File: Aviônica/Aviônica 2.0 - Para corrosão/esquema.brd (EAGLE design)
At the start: 128 x 64.1 mm, 15 parts, among them M1 WIRELESS-NRF24L01-PA-EXT

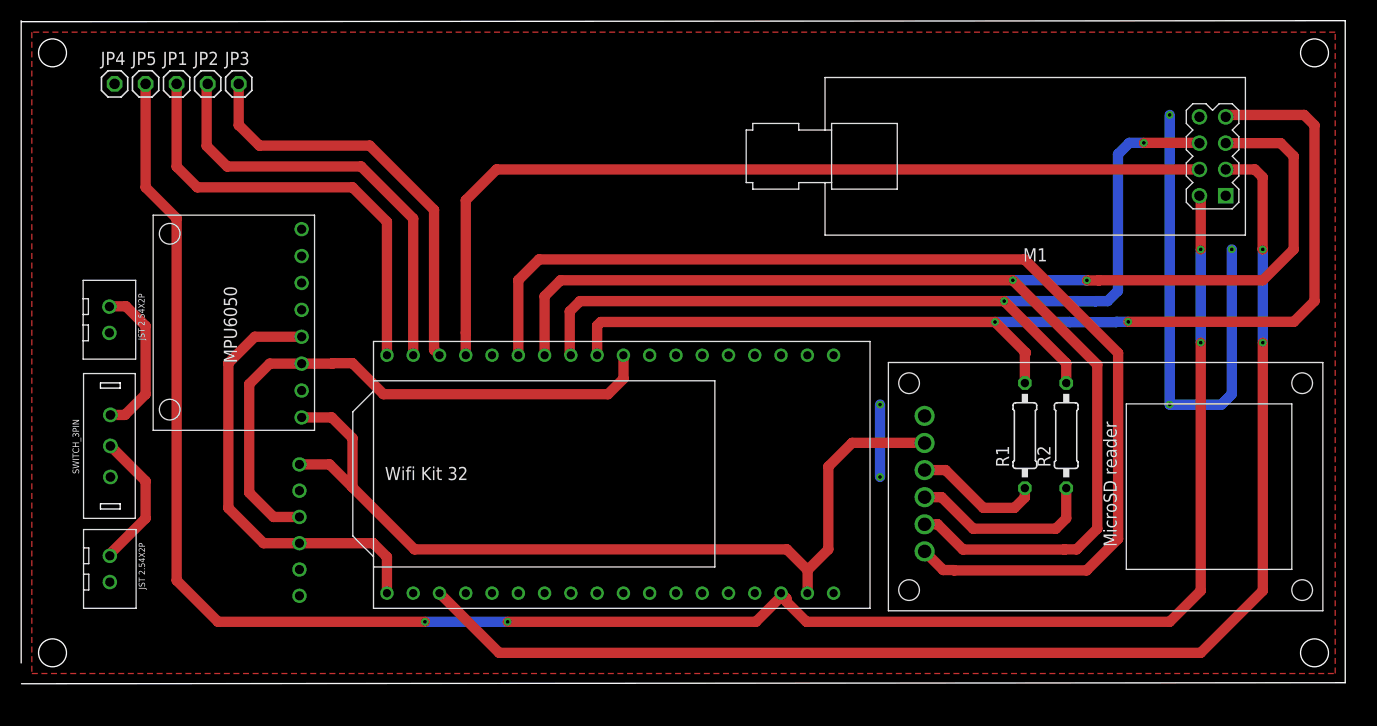
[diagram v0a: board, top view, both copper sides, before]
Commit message: Atualizando placas
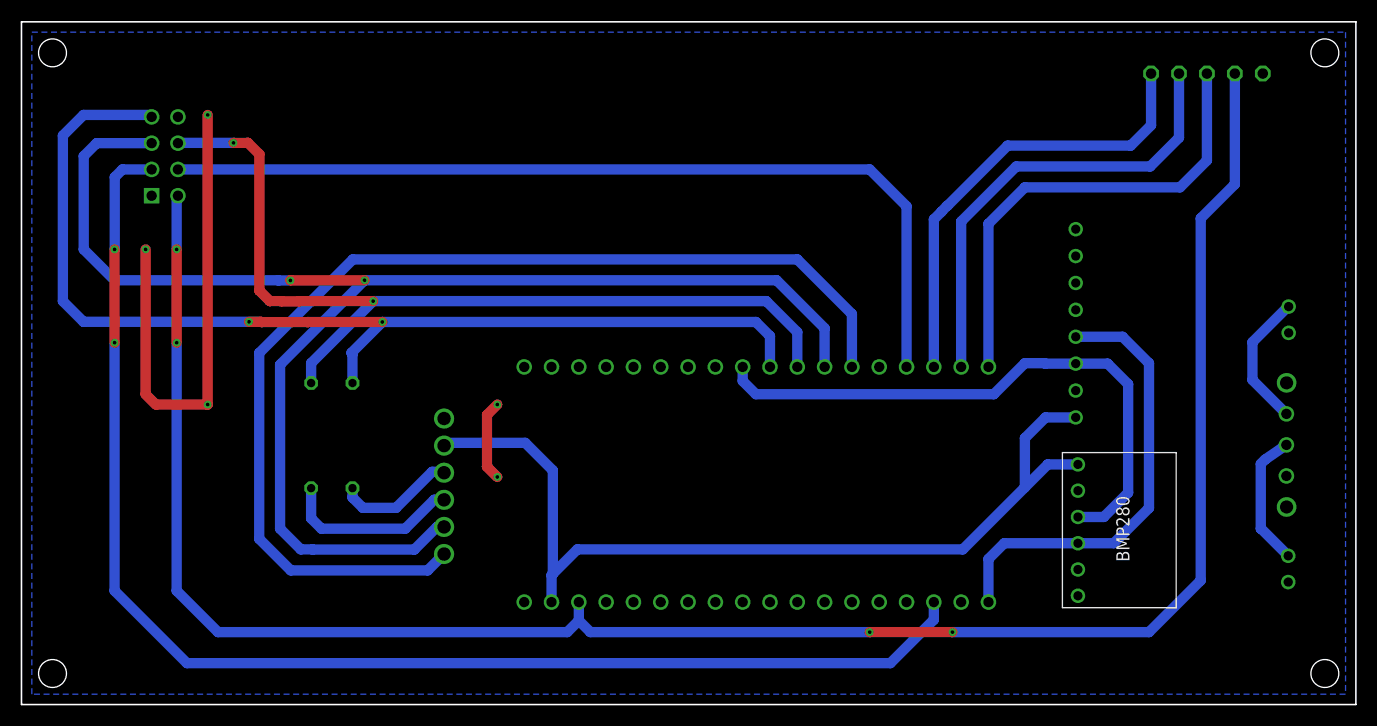
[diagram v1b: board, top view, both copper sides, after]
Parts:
- moved U$6 115.3 mm to (122.3, 21.1), flipped to the bottom
- moved U$7 114.0 mm to (122.5, 33.2), flipped to the bottom
- moved U$5 113.9 mm to (122.5, 9.11), flipped to the bottom
- moved JP4 111.0 mm to (120.0, 57.0), flipped to the bottom
- moved JP5 105.3 mm to (117.3, 57.0), flipped to the bottom
- moved JP1 99.6 mm to (114.6, 57.0), flipped to the bottom
- moved U$3 95.2 mm to (112.1, 32.7), flipped to the bottom
- moved JP2 93.9 mm to (111.9, 57.0), flipped to the bottom
- moved JP3 88.2 mm to (109.2, 57.0), flipped to the bottom
- moved U$1 87.5 mm to (108.2, 12.7), flipped to the top
- moved R2 73.0 mm to (28.0, 22.0), flipped to the bottom
- moved U$2 69.7 mm to (32.2, 17.0), flipped to the bottom
- moved M1 67.0 mm to (31.0, 49.0), flipped to the bottom
- moved R1 65.0 mm to (32.0, 22.0), flipped to the bottom
- moved U$4 13.8 mm to (61.8, 17.3), flipped to the bottom, turned to 90 degrees
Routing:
- net BUZZER: track 40.5 -> 44.0 mm
- net 3V3_1: track 87.2 -> 90.2 mm
- net SKIB2: track 42.1 -> 44.7 mm
- net SKIB1: track 43.4 -> 45.9 mm
- net N$1: track 108.5 -> 106.1 mm
- net SCLK: track 142.0 -> 139.6 mm
- net 3V3_2: track 192.1 -> 194.0 mm
- net VIN: track 15.1 -> 13.2 mm
- net MOSI: track 90.1 -> 89.0 mm
- net CE: track 128.3 -> 129.4 mm
- net MISO: track 106.5 -> 105.4 mm
- net MOSI_SD: track 18.3 -> 17.3 mm
- net SDA: track 42.9 -> 43.9 mm
- net MISO_SD: track 12.5 -> 11.7 mm
- net GND: track 55.4 -> 56.2 mm
- added copper zone on layer 16, net GND
- removed copper zone on layer 1, net GND
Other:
- board size 128 x 64.1 mm -> 129 x 66 mm
